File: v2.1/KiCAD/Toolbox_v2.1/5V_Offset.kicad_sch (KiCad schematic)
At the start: 22 parts, among them J26 Kinks_OUT_MAX, J27 Kinks_IN_A, J28 Kinks_IN_B, J29 Kinks_OUT_MIN, U6 TL074, U7 TL074

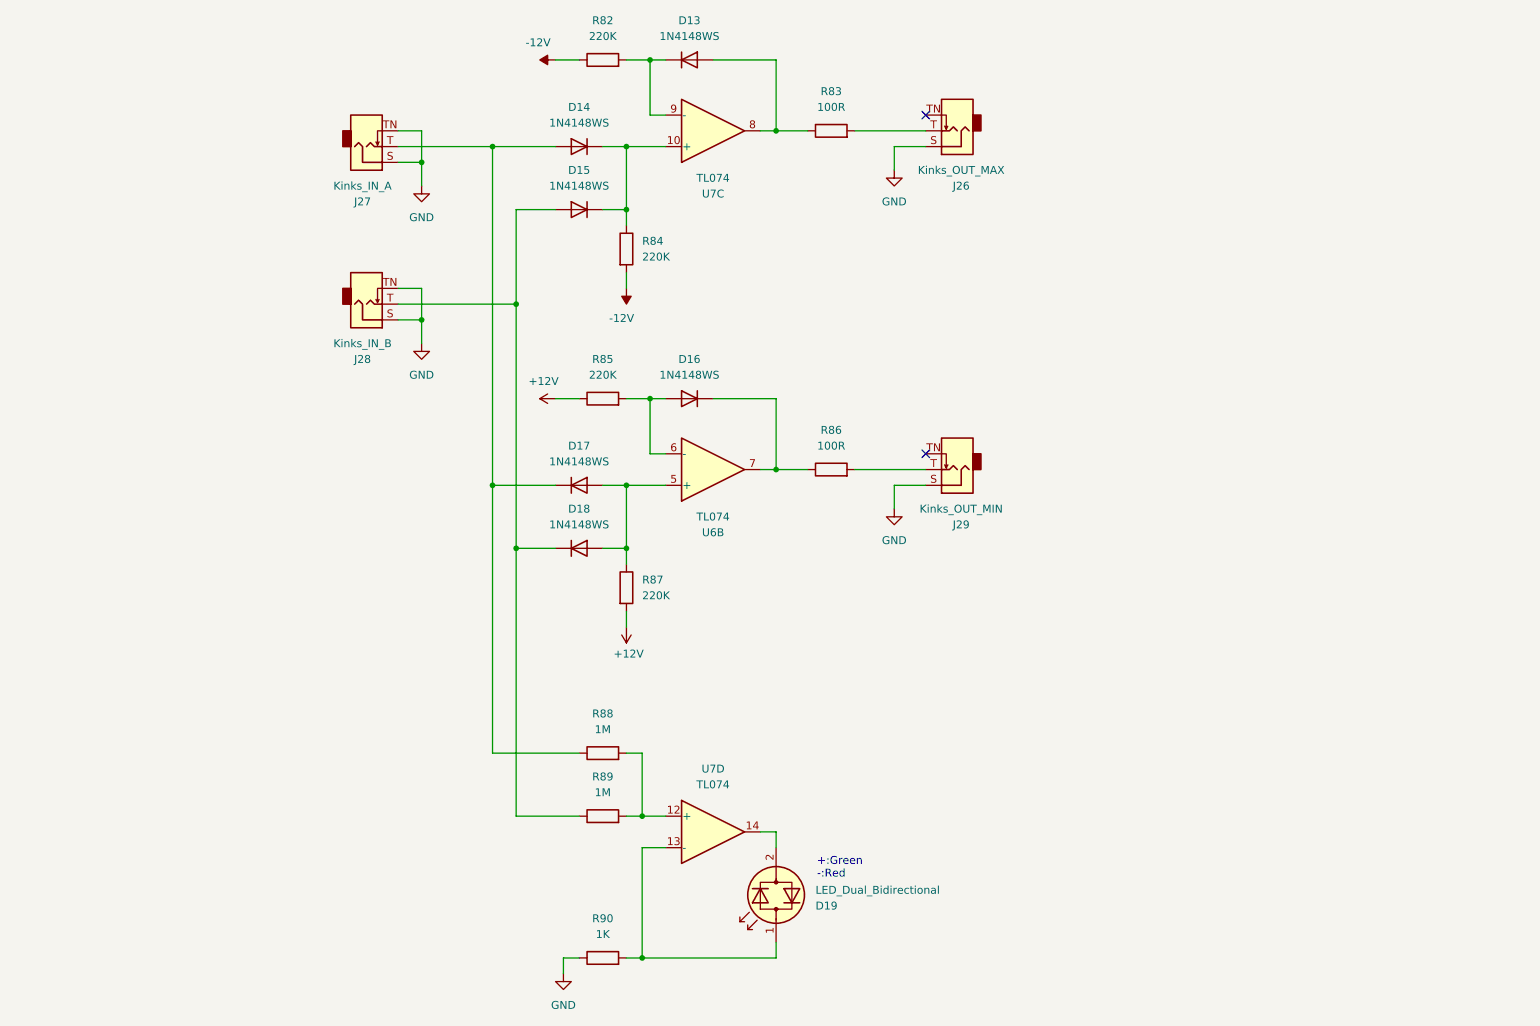
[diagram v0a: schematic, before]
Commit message: v2.1 Update
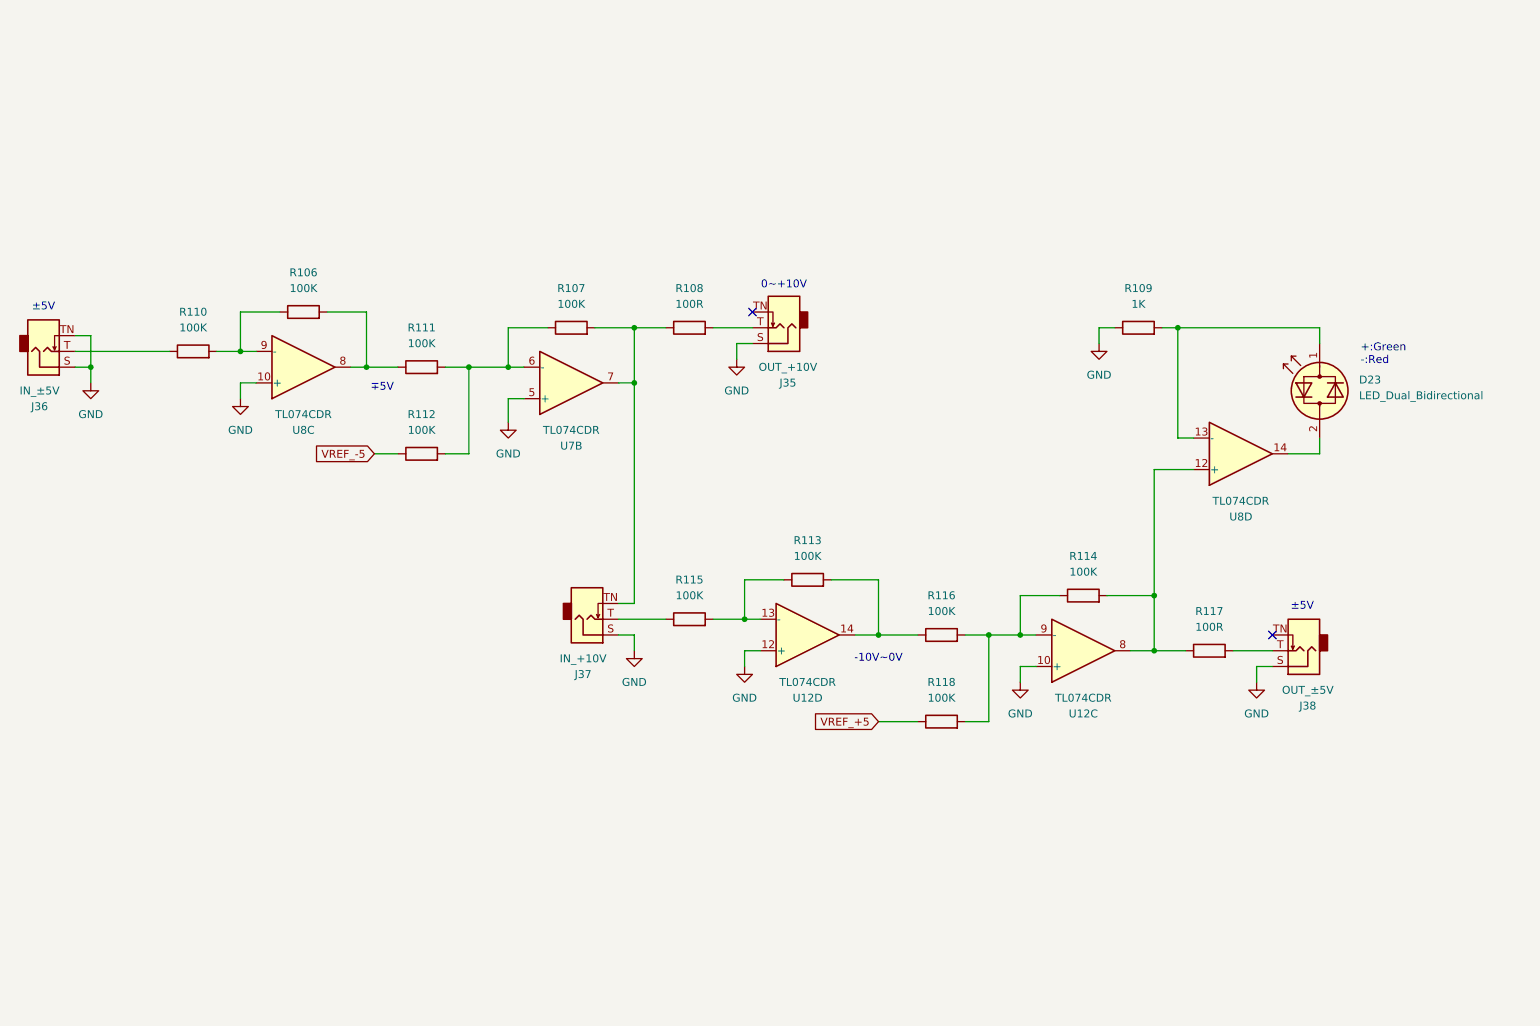
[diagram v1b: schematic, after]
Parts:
- removed D13, D14, D15, D16, D17, D18: 1N4148WS, Diode_SMD:D_SOD-323, symbol Diode:1N4148WS
- removed D19: LED_Dual_Bidirectional, LED_THT:LED_D3.0mm, symbol Device:LED_Dual_Bidirectional
- removed J26: Kinks_OUT_MAX, kat_eurorack:AudioJack_PJ301M-12, symbol Connector_Audio:AudioJack2_SwitchT
- removed J27: Kinks_IN_A, kat_eurorack:AudioJack_PJ301M-12, symbol Connector_Audio:AudioJack2_SwitchT
- removed J28: Kinks_IN_B, kat_eurorack:AudioJack_PJ301M-12, symbol Connector_Audio:AudioJack2_SwitchT
- removed J29: Kinks_OUT_MIN, kat_eurorack:AudioJack_PJ301M-12, symbol Connector_Audio:AudioJack2_SwitchT
- removed R82, R84, R85, R87: 220K, Resistor_SMD:R_0402_1005Metric, symbol Device:R
- removed R83, R86: 100R, Resistor_SMD:R_0402_1005Metric, symbol Device:R
- removed R88, R89: 1M, Resistor_SMD:R_0402_1005Metric, symbol Device:R
- removed R90: 1K, Resistor_SMD:R_0402_1005Metric, symbol Device:R
- removed U6, U7: TL074, Package_SO:TSSOP-14_4.4x5mm_P0.65mm, symbol Amplifier_Operational:TL074
- added D23: LED_Dual_Bidirectional, LED_THT:LED_D3.0mm, symbol Device:LED_Dual_Bidirectional
- added J35: OUT_+10V, kat_eurorack:AudioJack_PJ301M-12, symbol Connector_Audio:AudioJack2_SwitchT
- added J36: IN_±5V, kat_eurorack:AudioJack_PJ301M-12, symbol Connector_Audio:AudioJack2_SwitchT
- added J37: IN_+10V, kat_eurorack:AudioJack_PJ301M-12, symbol Connector_Audio:AudioJack2_SwitchT
- added J38: OUT_±5V, kat_eurorack:AudioJack_PJ301M-12, symbol Connector_Audio:AudioJack2_SwitchT
- added R106, R107, R110, R111, R112, R113, R114, R115, R116, R118: 100K, Resistor_SMD:R_0402_1005Metric, symbol Device:R
- added R108, R117: 100R, Resistor_SMD:R_0402_1005Metric, symbol Device:R
- added R109: 1K, Resistor_SMD:R_0402_1005Metric, symbol Device:R
- added U12, U7, U8: TL074CDR, Package_SO:SOIC-14_3.9x8.7mm_P1.27mm, symbol Amplifier_Operational:TL074
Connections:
- net GND: now also J35.S, J36.S, J36.TN, J37.S, J38.S, R109.1, U12.10 (+), U12.12 (+), U7.5 (+), U8.10 (+)
- new net: J38.T, R117.2
- new net: R107.1, R111.2, R112.2, U7.6 (-)
- new net: J37.TN, R107.2, R108.1, U7.7
- new net: R113.1, R115.2, U12.13 (-)
- new net: R113.2, R116.1, U12.14
- new net: R114.1, R116.2, R118.2, U12.9 (-)
- new net: R114.2, R117.1, U12.8, U8.12 (+)
- new net: D23.1 (KA), R109.2, U8.13 (-)
- new net: D23.2 (AK), U8.14
- new net: R106.2, R111.1, U8.8
- new net: J36.T, R110.1
- new net: R106.1, R110.2, U8.9 (-)
- new net: J37.T, R115.1
- new net: J35.T, R108.2
- new net VREF_+5: R118.1
- new net VREF_-5: R112.1
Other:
- note added: "-10V~0V"
- note added: "0~+10V"
- note added: "±5V"
- note added: "∓5V"
- title: Analog AND/OR -> ±5V Offset
